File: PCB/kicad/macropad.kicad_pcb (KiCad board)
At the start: 2 copper layers, 99.8 x 92 mm, 77 parts, among them J1 OLED_128x32, J2 4P4C, SW1 RESET_Push, SW2 RotaryEncoder_Switch, SW3 RotaryEncoder_Switch, SW4 RotaryEncoder_Switch, SW5 Soft_Push, SW6 Soft_Push, SW7 Soft_Push, U1 5-Way Nav, U2 NOT Gate, U3 ON/OFF

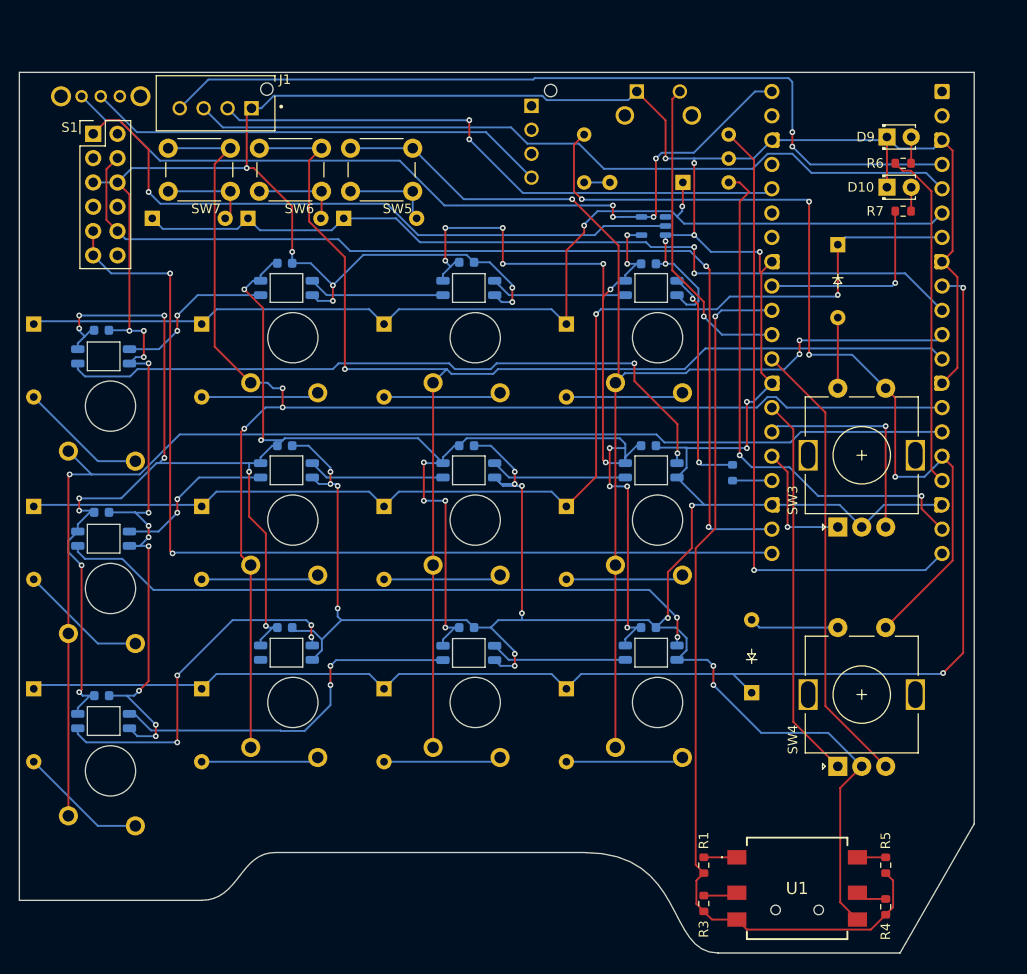
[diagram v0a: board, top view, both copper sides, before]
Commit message: Routed PCB
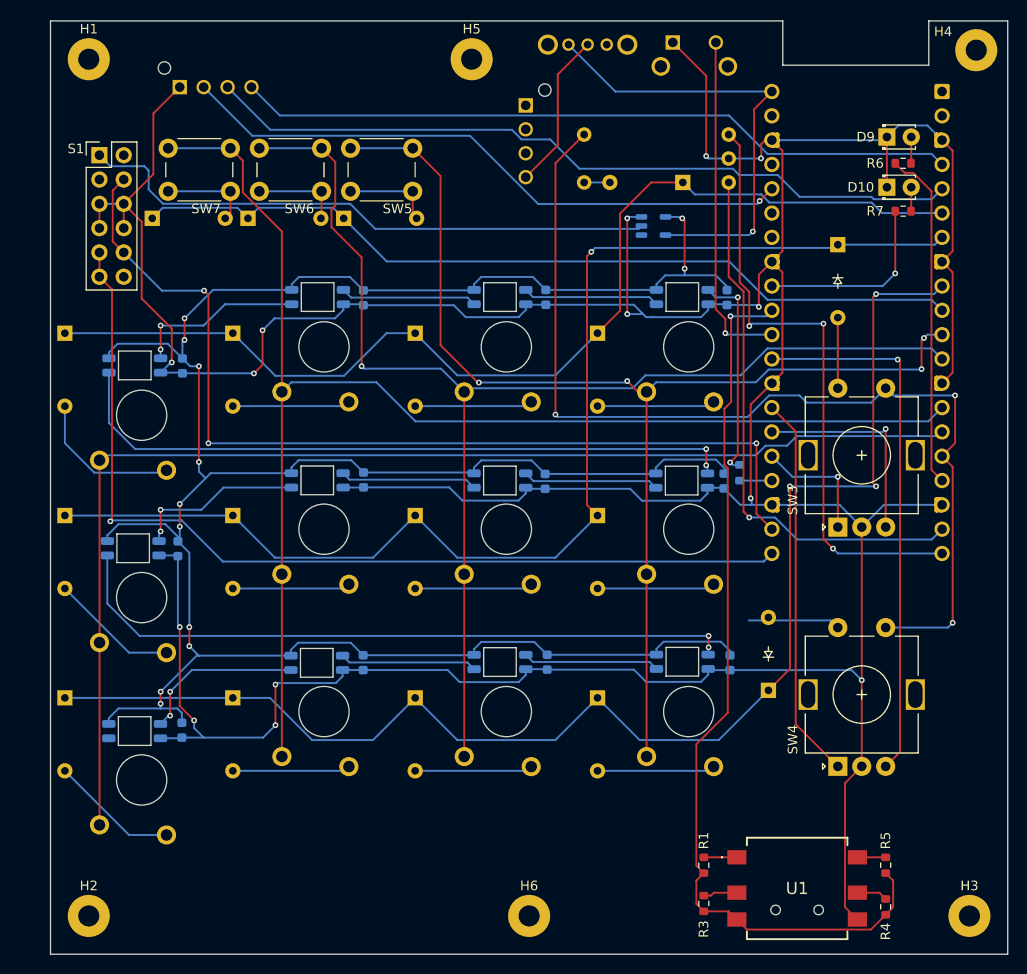
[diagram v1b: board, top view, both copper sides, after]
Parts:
- added H1: Pad, MountingHole:MountingHole_2.2mm_M2_Pad, F.Cu at (147.8, 56.6)
- added H2: Pad, MountingHole:MountingHole_2.2mm_M2_Pad, F.Cu at (147.8, 146.1)
- added H3: Pad, MountingHole:MountingHole_2.2mm_M2_Pad, F.Cu at (239.8, 146.1)
- added H4: Pad, MountingHole:MountingHole_2.2mm_M2_Pad, F.Cu at (240.5, 55.7)
- added H5: Pad, MountingHole:MountingHole_2.2mm_M2_Pad, F.Cu at (187.8, 56.6)
- added H6: Pad, MountingHole:MountingHole_2.2mm_M2_Pad, F.Cu at (193.8, 146.1)
- J1: moved to B.Cu
- moved U3 51.1 mm to (199.9, 55.1)
- moved D13 23.1 mm to (171.6, 119.7)
- moved D14 17.8 mm to (152.5, 126.8)
- moved C9 9.27 mm to (214.7, 119.7), turned to -90 degrees
- moved C4 9.24 mm to (157.5, 88.7), turned to -90 degrees
- moved C10 9.16 mm to (195.6, 119.6), turned to -90 degrees
- moved C12 9.12 mm to (157.5, 126.7), turned to -90 degrees
- moved C2 9.04 mm to (195.5, 81.5), turned to -90 degrees
- moved C6 9.01 mm to (195.4, 100.7), turned to -90 degrees
- moved C11 8.98 mm to (176.4, 119.7), turned to -90 degrees
- moved C7 8.97 mm to (176.5, 100.6), turned to -90 degrees
- moved C3 8.97 mm to (176.4, 81.6), turned to -90 degrees
- moved C1 8.93 mm to (214.4, 81.5), turned to -90 degrees
- moved C8 8.83 mm to (157.1, 107.8), turned to -90 degrees
- moved C5 8.70 mm to (214.1, 100.7), turned to -90 degrees
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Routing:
- net GND: track 529.4 -> 461.4 mm, vias 39 -> 14
- net +5V: track 86.9 -> 48.5 mm, vias 4 -> 1
- net Net-(J2-V): track 48.5 -> 16.5 mm
- net Net-(D12-DOUT): track 39.0 -> 14.3 mm, vias 2 -> 0
- net Net-(D1-VDD): track 286.9 -> 265.1 mm, vias 29 -> 12
- net Net-(D13-DOUT): track 37.1 -> 17.4 mm, vias 4 -> 2
- net SDA: track 88.6 -> 75.5 mm, vias 2 -> 0
- net ENC SW: track 93.7 -> 106.5 mm, vias 4 -> 3
- net B2: track 47.5 -> 56.4 mm, vias 0 -> 1
- net Net-(U2-A): track 68.4 -> 61.1 mm, vias 1 -> 0
- net ROW1: track 122.3 -> 128.4 mm, vias 2 -> 1
- net COL3: track 132.8 -> 128.1 mm, vias 1 -> 0
- net DP4T 2: track 105.7 -> 101.6 mm, vias 2 -> 3
- net COL2: track 147.4 -> 143.9 mm, vias 3 -> 0
- net DP4T 1: track 103.4 -> 100.0 mm, vias 2 -> 1
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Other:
- board size 99.8 x 92 mm -> 100 x 97.5 mm
